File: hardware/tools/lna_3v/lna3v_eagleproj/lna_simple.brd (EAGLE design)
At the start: 27.9 x 16.2 mm, 11 parts, among them U1 BGA2801, X1 SMA-142-0701-801/806, X2 SMA-142-0701-801/806

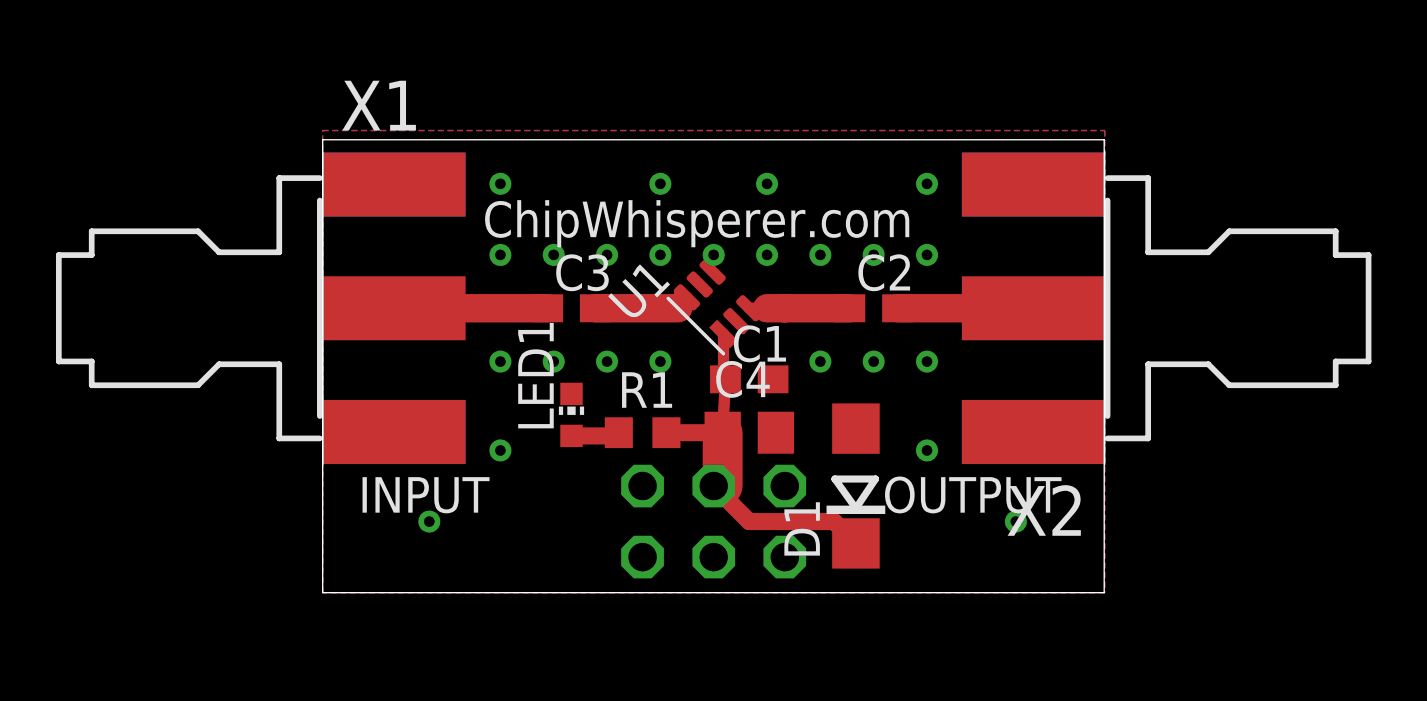
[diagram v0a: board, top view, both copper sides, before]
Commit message: HW: Update LNA PCB to Latest beta, not tested in HW yet
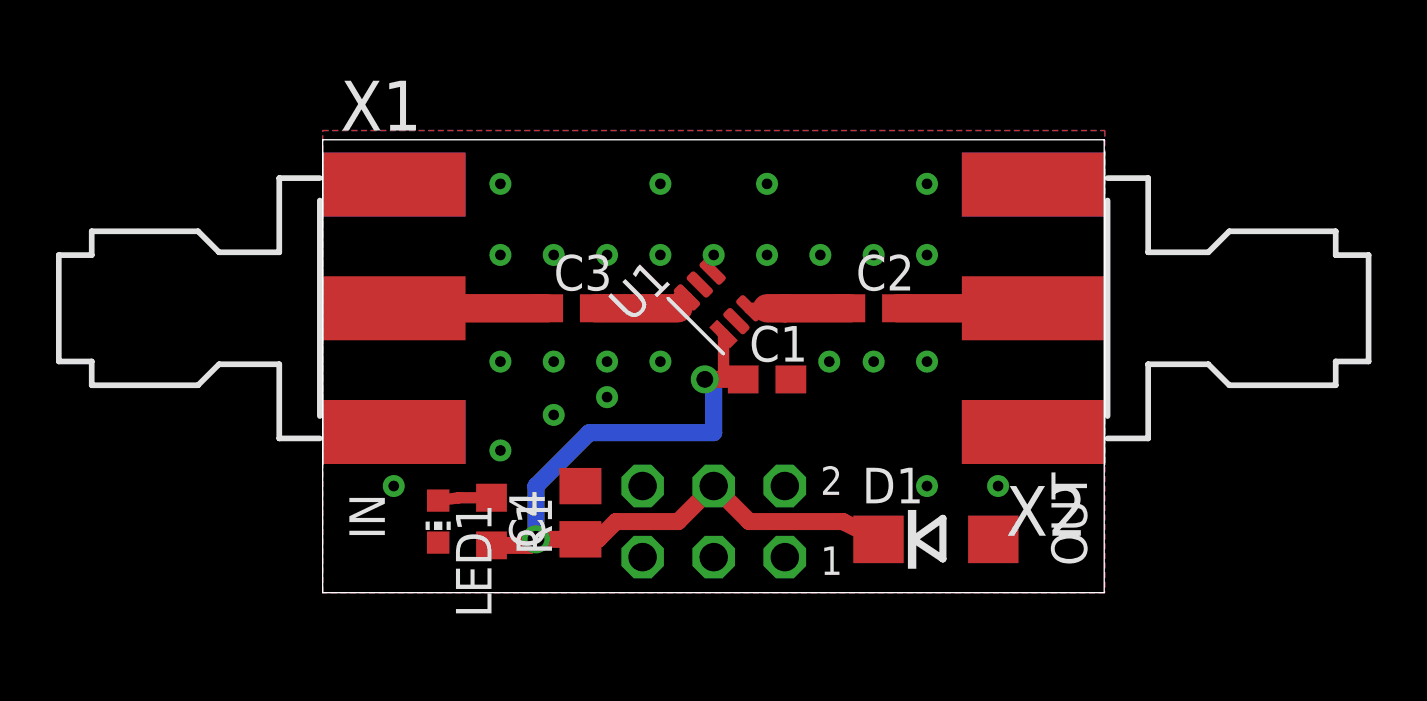
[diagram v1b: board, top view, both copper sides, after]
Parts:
- moved C4 6.68 mm to (24.4, 19.4), turned to 90 degrees
- moved R1 6.26 mm to (21.3, 19.1), turned to 270 degrees
- moved LED1 6.10 mm to (19.4, 19.1), turned to 180 degrees
- moved D1 3.43 mm to (37.1, 18.4), turned to 0 degrees
- moved C1 0.63 mm to (31.1, 24.1)
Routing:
- net AVCC: track 14.0 -> 30.2 mm, vias 0 -> 2
- net AGND: vias 24 -> 26
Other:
- board text added: "+20dB"
- board text added: "1"
- board text added: "2"
- board text added: "3.3V"
- board text added: "4:+3.3V"
- board text added: "5"
- board text added: "6"
- board text added: "6:GND"
- board text added: "GND"
- board text added: "IN"
- board text added: "Inc."
- board text added: "NPCB-LNA-02"
- board text added: "NewAE"
- board text added: "OUT"
- board text added: "Technology"
- board text removed: "INPUT"
- board text removed: "OUTPUT"
